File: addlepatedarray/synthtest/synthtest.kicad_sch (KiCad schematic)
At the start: 72 parts, among them J1 RF0A+, J2 RF0A-, J3 RF0B-, J4 RF0B+, J5 RF1A-, J6 RF1B-, J7 RF1A+, J8 RF1B+, J9 REF, U1 ADF4351, U2 ADF4351, U4 CH32V003FxUx, U6 LDL1117-33, Y1 TG-5006CG-12H 26.0000M3

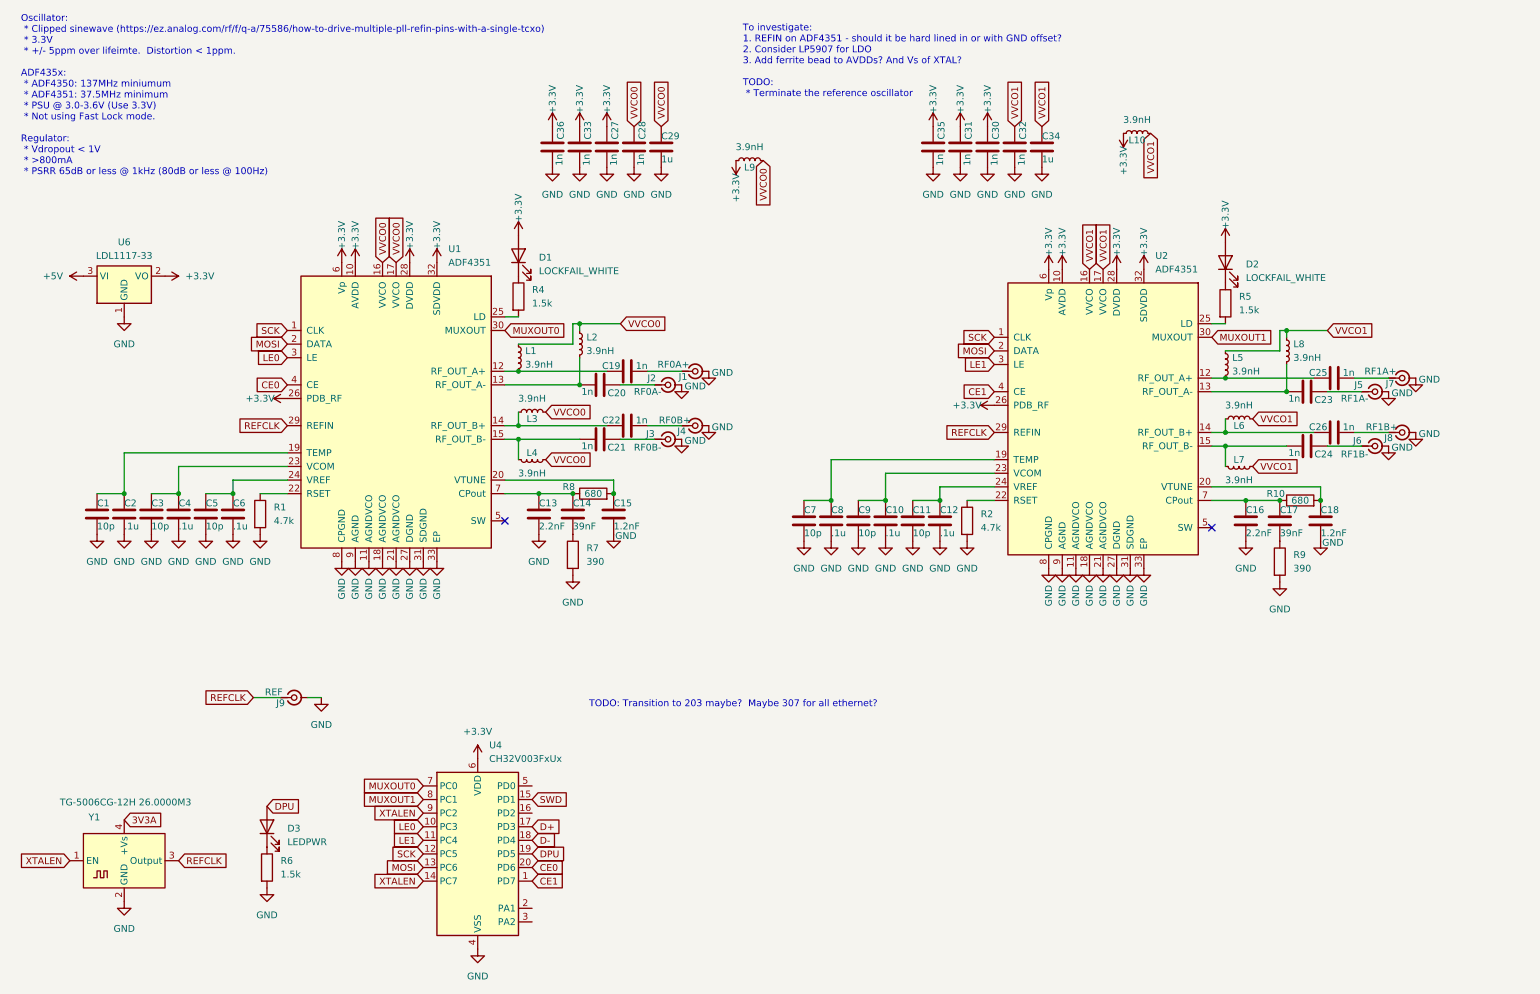
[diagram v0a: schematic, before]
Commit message: Bump disign!
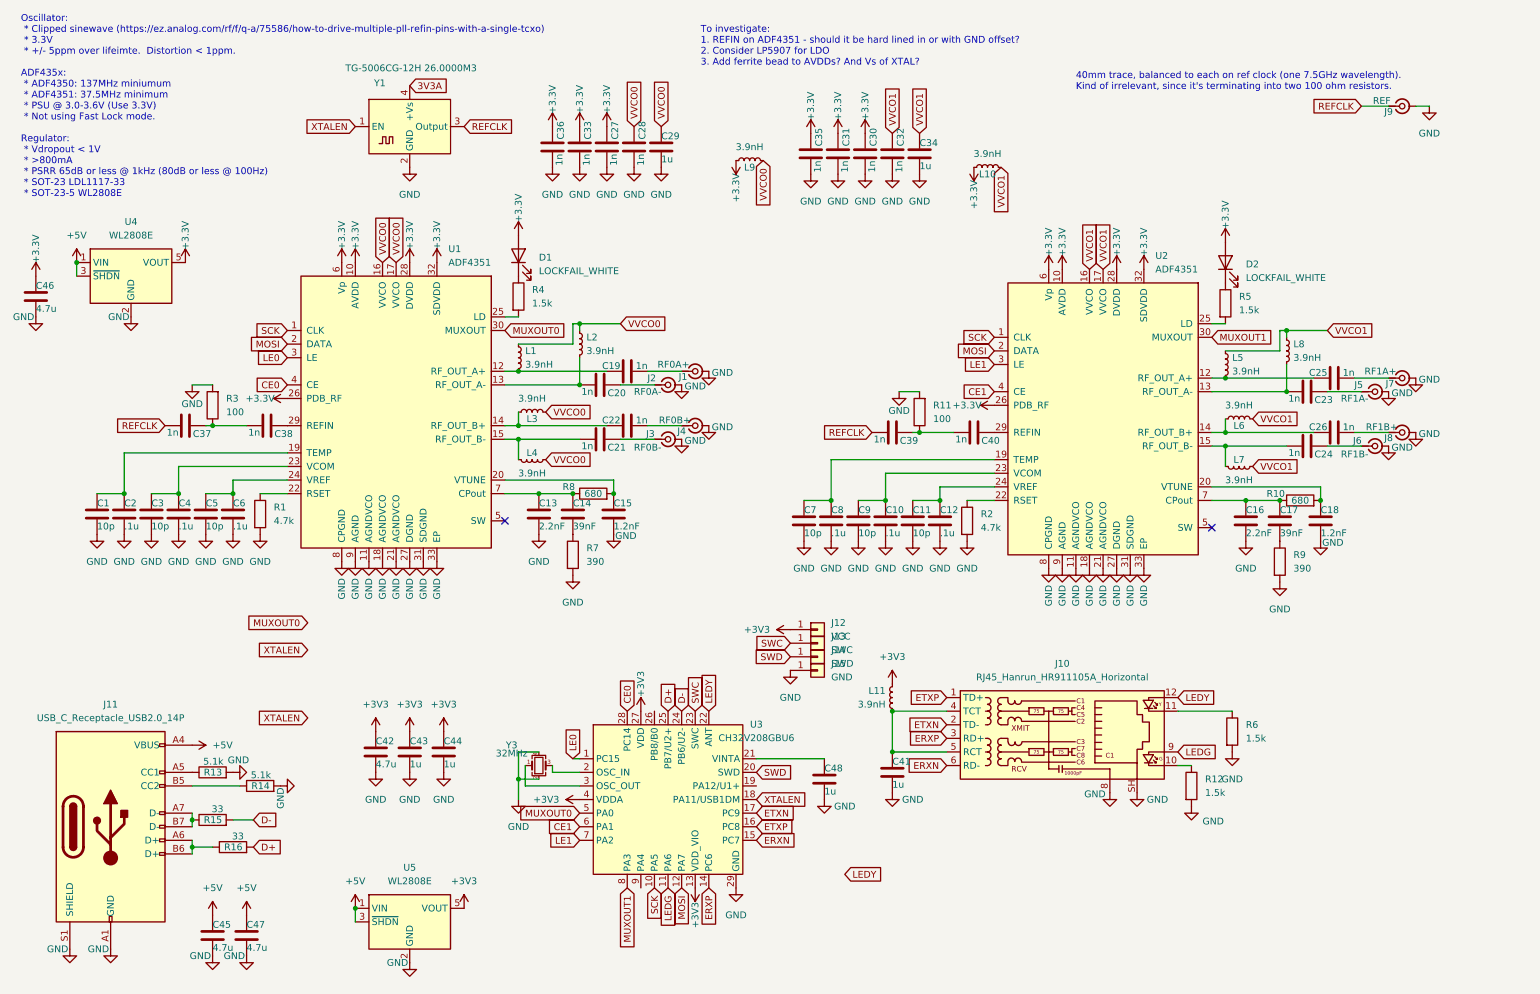
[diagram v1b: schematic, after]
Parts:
- removed D3: LEDPWR, LED_SMD:LED_0603_1608Metric, symbol Device:LED
- removed U4: CH32V003FxUx, Package_DFN_QFN:QFN-20-1EP_3x3mm_P0.4mm_EP1.65x1.65mm, symbol MCU_WCH_CH32V0:CH32V003FxUx
- removed U6: LDL1117-33, Package_TO_SOT_SMD:SOT-223-3_TabPin2, symbol Regulator_Linear:AMS1117-3.3
- added C37, C38, C39, C40: 1n, Capacitor_SMD:C_0402_1005Metric, symbol Device:C
- added C41, C43, C44, C48: 1u, Capacitor_SMD:C_0402_1005Metric, symbol Device:C
- added C42, C45, C46, C47: 4.7u, Capacitor_SMD:C_0603_1608Metric, symbol Device:C
- added J10: RJ45_Hanrun_HR911105A_Horizontal, cnhardware:HR915310A-RJ45-INTEGRATED-10MBIT, symbol Connector:RJ45_Hanrun_HR911105A_Horizontal
- added J11: USB_C_Receptacle_USB2.0_14P, Connector_USB:USB_C_Receptacle_G-Switch_GT-USB-7051x, symbol Connector:USB_C_Receptacle_USB2.0_14P
- added J12: VCC, TestPoint:TestPoint_Pad_D1.0mm, symbol Connector_Generic:Conn_01x01
- added J13: SWC, TestPoint:TestPoint_Pad_D1.0mm, symbol Connector_Generic:Conn_01x01
- added J14: SWD, TestPoint:TestPoint_Pad_D1.0mm, symbol Connector_Generic:Conn_01x01
- added J15: GND, TestPoint:TestPoint_Pad_D1.0mm, symbol Connector_Generic:Conn_01x01
- added L11: 3.9nH, Inductor_SMD:L_0402_1005Metric, symbol Device:L_Small
- added R11, R3: 100, Resistor_SMD:R_0402_1005Metric, symbol Device:R
- added R12: 1.5k, cnhardware:R_0402_1005Metric_COMPACT, symbol Device:R
- added R13, R14: 5.1k, Resistor_SMD:R_0402_1005Metric, symbol Device:R
- added R15, R16: 33, Resistor_SMD:R_0402_1005Metric, symbol Device:R
- added U3: CH32V208GBU6, Package_DFN_QFN:QFN-28-1EP_4x4mm_P0.45mm_EP2.6x2.6mm, symbol cnhardware:CH32V208GBU6
- added U4, U5: WL2808E, Package_TO_SOT_SMD:SOT-23-5, symbol Regulator_Linear:MCP1802x-xx02xOT
- added Y3: 32MHz, Crystal:Crystal_SMD_2016-4Pin_2.0x1.6mm, symbol Device:Crystal_GND24_Small
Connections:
- net +3.3V: now also C46.1, U4.5 (VOUT)
- net +5V: now also C45.1, C47.1, J11.A4 (VBUS), J11.A9 (VBUS), J11.B4 (VBUS), J11.B9 (VBUS), U4.1 (VIN), U4.3 (~{SHDN}), U5.1 (VIN), U5.3 (~{SHDN})
- net CE0: now also U3.28 (PC14)
- net CE1: now also U3.6 (PA1)
- net D+: now also R16.2, U3.25 (PB7/U2+)
- net D-: now also R15.2, U3.24 (PB6/U2-)
- net GND: now also C41.2, C42.2, C43.2, C44.2, C45.2, C46.2, C47.2, C48.2, J10.8, J10.SH, J11.A1 (GND), J11.A12 (GND), J11.B1 (GND), J11.B12 (GND), J11.S1 (SHIELD), J15.1 (Pin_1), R11.2, R12.2, R13.2, R14.2, R3.2, U3.29 (GND), U4.2 (GND), U5.2 (GND), Y3.2, Y3.4
- net LE0: now also U3.1 (PC15)
- net LE1: now also U3.7 (PA2)
- net MOSI: now also U3.12 (PA7)
- net MUXOUT0: now also U3.5 (PA0)
- net MUXOUT1: now also U3.8 (PA3)
- net REFCLK: now also C37.1, C39.1; no longer U1.29 (REFIN), U2.29 (REFIN)
- net SCK: now also U3.10 (PA5)
- net SWD: now also J14.1 (Pin_1), U3.20 (SWD)
- net XTALEN: now also U3.18 (PA11/USB1DM)
- net at R6.1: now also J10.11
- new net: J11.A5 (CC1), R13.1
- new net: C48.1, U3.21 (VINTA)
- new net: J10.10, R12.1
- new net: C41.1, J10.4 (TCT), J10.5 (RCT), L11.2
- new net: J11.B5 (CC2), R14.1
- new net: J11.A6 (D+), J11.B6 (D+), R16.1
- new net: J11.A7 (D-), J11.B7 (D-), R15.1
- new net: C38.2, U1.29 (REFIN)
- new net: C39.2, C40.1, R11.1
- new net: C40.2, U2.29 (REFIN)
- new net: U3.3 (OSC_OUT), Y3.1
- new net: U3.2 (OSC_IN), Y3.3
- new net: C37.2, C38.1, R3.1
- new net +3V3: C42.1, C43.1, C44.1, J12.1 (Pin_1), L11.1, U3.13 (VDD_VIO), U3.27 (VDD), U3.4 (VDDA), U5.5 (VOUT)
- new net ERXN: J10.6 (RD-), U3.15 (PC7)
- new net ERXP: J10.3 (RD+), U3.14 (PC6)
- new net ETXN: J10.2 (TD-), U3.17 (PC9)
- new net ETXP: J10.1 (TD+), U3.16 (PC8)
- new net LEDG: J10.9, U3.11 (PA6)
- new net LEDY: J10.12, U3.22 (ANT)
- new net SWC: J13.1 (Pin_1), U3.23 (SWC)
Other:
- note added: "40mm trace, balanced to each on ref clock (one 7.5GHz wavelength). Kind of irrelevant, since it's terminating into two 100 ohm resistors."
- note added: "Oscillator: * Clipped sinewave (https://ez.analog.com/rf/f/q-a/75586/how-to-drive-multiple-pll-refin-pins-with-a-single-tcxo) * 3.3V * +/- 5ppm over lifeimte. Distortion < 1ppm. ADF435x: * ADF4350: 137MHz miniumum * ADF4351: 37.5MHz minimum * PSU @ 3.0-3.6V (Use 3.3V) * Not using Fast Lock mode. Regulator: * Vdropout < 1V * >800mA * PSRR 65dB or less @ 1kHz (80dB or less @ 100Hz) * SOT-23 LDL1117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"
- note added: "To investigate: 1. REFIN on ADF4351 - should it be hard lined in or with GND offset? 2. Consider LP5907 for LDO 3. Add ferrite bead to AVDDs? And Vs of XTAL?"
- note removed: "Oscillator: * Clipped sinewave (https://ez.analog.com/rf/f/q-a/75586/how-to-drive-multiple-pll-refin-pins-with-a-single-tcxo) * 3.3V * +/- 5ppm over lifeimte. Distortion < 1ppm. ADF435x: * ADF4350: 137MHz miniumum * ADF4351: 37.5MHz minimum * PSU @ 3.0-3.6V (Use 3.3V) * Not using Fast Lock mode. Regulator: * Vdropout < 1V * >800mA * PSRR 65dB or less @ 1kHz (80dB or less @ 100Hz)"
- note removed: "TODO: Transition to 203 maybe? Maybe 307 for all ethernet?"
- note removed: "To investigate: 1. REFIN on ADF4351 - should it be hard lined in or with GND offset? 2. Consider LP5907 for LDO 3. Add ferrite bead to AVDDs? And Vs of XTAL? TODO: * Terminate the reference oscillator"
- moved on the sheet: C30, C31, C32, C34, C35, J9, L10, R6, Y1
